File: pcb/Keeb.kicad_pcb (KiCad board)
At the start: 2 copper layers, 142.6 x 98.1 mm, 96 parts, among them J1 TRRS_SJ1-42514, J2 TRRS_SJ1-42514, K00 KEYSW, K01 KEYSW, K02 KEYSW, K03 KEYSW, K04 KEYSW, K05 KEYSW, K10 KEYSW, K11 KEYSW, K12 KEYSW, K13 KEYSW, K14 KEYSW, K15 KEYSW, K20 KEYSW, K21 KEYSW, K22 KEYSW, K23 KEYSW, K24 KEYSW, K25 KEYSW, K26 KEYSW, K30 KEYSW, K31 KEYSW, K32 KEYSW, K33 KEYSW, K34 KEYSW, K35 KEYSW, K36 KEYSW, SW1 SW_RST, U1 ATMEGA32U4, U2 PI6ULS5V9511AWEX_I2C_HotSwap, U3 MCP23017_SO, X1 XTAL_GND

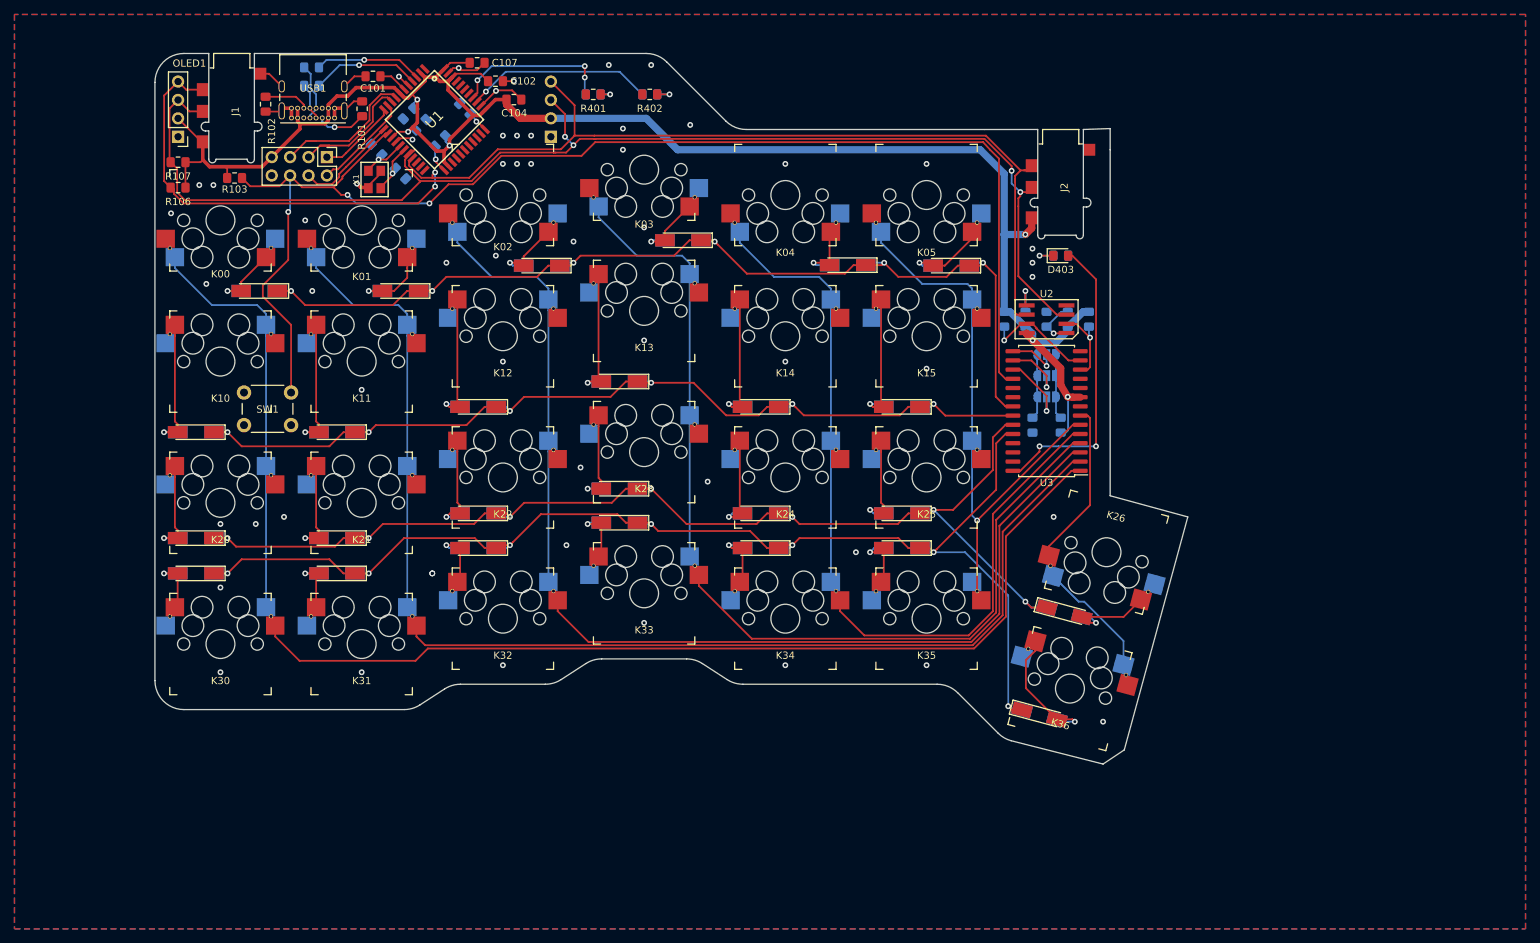
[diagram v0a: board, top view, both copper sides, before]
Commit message: restarted layout
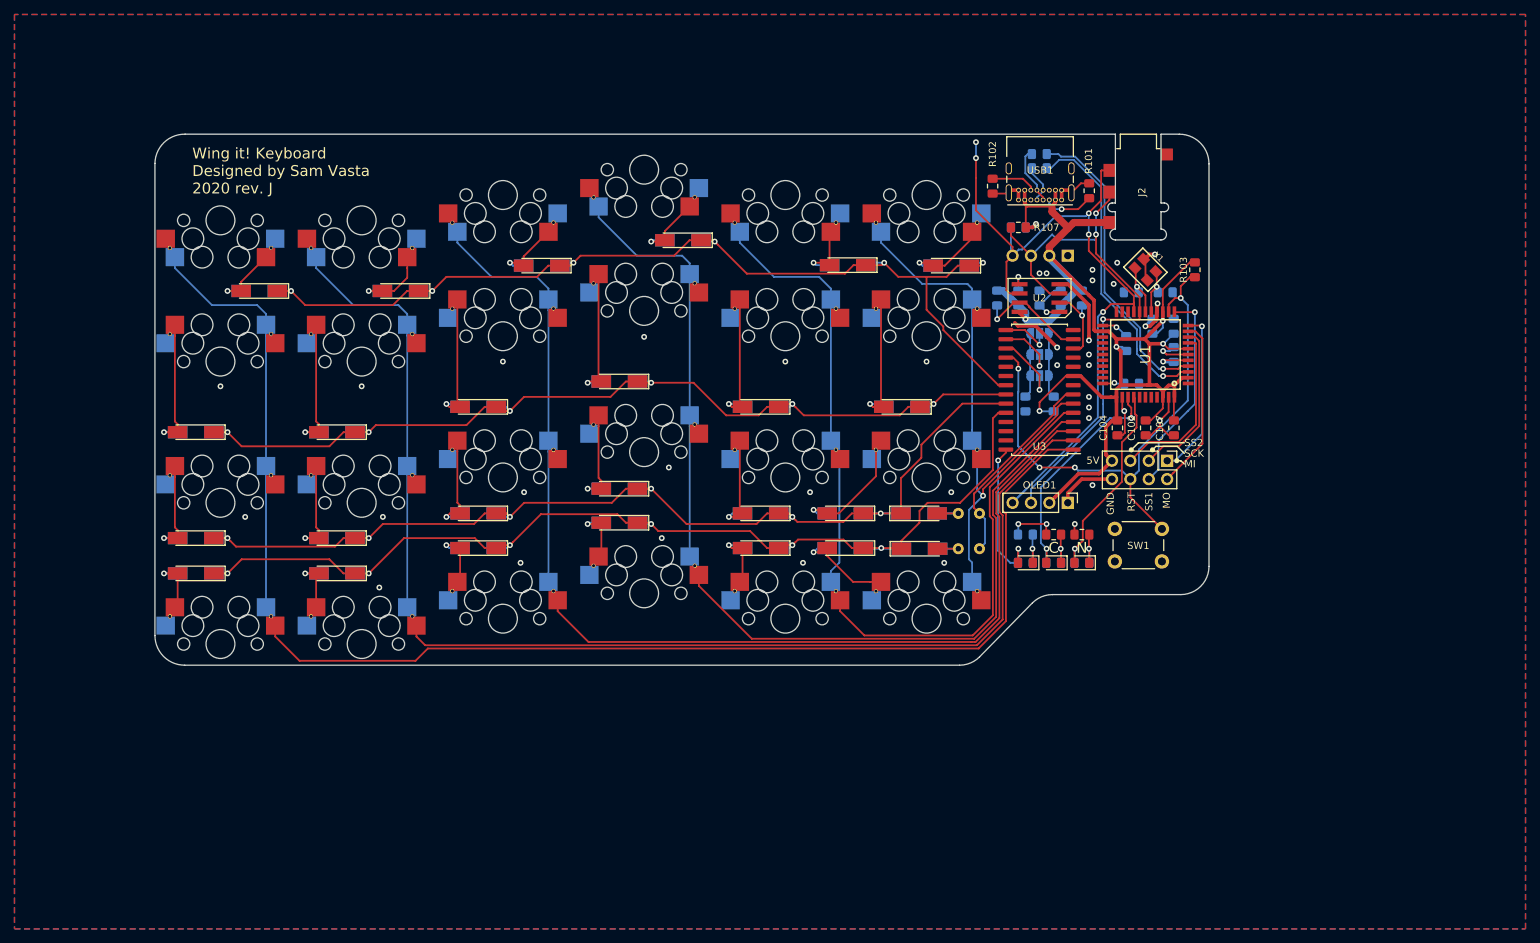
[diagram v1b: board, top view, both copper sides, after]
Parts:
- removed J1: TRRS_SJ1-42514, SVastaCustomParts:3.5mm_Cut_out
- removed JP0, JP1, JP2: SolderJumper_3_Open, Jumper:SolderJumper-3_P1.3mm_Open_RoundedPad1.0x1.5mm
- removed the OLED1 at (201.1, 43.2)
- removed the OLED1 at (252.5, 43.2)
- added 1: SolderJumper_3_Open, Jumper:SolderJumper-3_P1.3mm_Open_RoundedPad1.0x1.5mm, B.Cu at (320.0, 70.4)
- added 2: SolderJumper_3_Open, Jumper:SolderJumper-3_P1.3mm_Open_RoundedPad1.0x1.5mm, B.Cu at (320.0, 73.3)
- added 4: SolderJumper_3_Open, Jumper:SolderJumper-3_P1.3mm_Open_RoundedPad1.0x1.5mm, B.Cu at (320.0, 76.2)
- added D401: CAPS, LED_SMD:LED_0805_2012Metric_Pad1.15x1.40mm_HandSolder, F.Cu at (325.9, 102.0)
- added D402: NUM, LED_SMD:LED_0805_2012Metric_Pad1.15x1.40mm_HandSolder, F.Cu at (322.0, 102.0)
- added D403: CONN, LED_SMD:LED_0805_2012Metric_Pad1.15x1.40mm_HandSolder, B.Cu at (318.1, 102.0)
- added G***: LOGO, SVastaCustomParts:wing_it_400dpi, B.Cu at (215.2, 48.9)
- added OLED1: Conn_01x04, Connector_PinHeader_2.54mm:PinHeader_1x04_P2.54mm_Vertical, B.Cu at (323.9, 59.6)
- added OLED1: Conn_01x04, Connector_PinHeader_2.54mm:PinHeader_1x04_P2.54mm_Vertical, F.Cu at (323.9, 93.8)
- C101, R106: moved to B.Cu
- K26, K36: footprint SVastaCustomParts:Kailh_socket_reversible -> SVastaCustomParts:switch_off_board
- moved R103 133.2 mm to (341.5, 61.6), turned to 270 degrees
- moved SPI1 123.4 mm to (337.6, 87.9)
- moved SW1 118.2 mm to (333.7, 99.6)
- moved C101 117.0 mm to (338.5, 73.3), turned to 270 degrees
- moved R107 116.4 mm to (317.1, 55.7)
- moved R106 116.2 mm to (317.1, 55.7)
- moved C108 110.7 mm to (337.4, 64.7), turned to 0 degrees
- moved C106 109.7 mm to (338.5, 69.4), turned to 90 degrees
- moved C107 108.6 mm to (338.6, 83.4), turned to 270 degrees
- moved X1 107.2 mm to (334.6, 61.6), turned to 135 degrees
- moved C105 104.8 mm to (335.6, 69.4), turned to 90 degrees
- moved U1 103.4 mm to (334.6, 73.3), turned to 180 degrees
- moved C109 102.2 mm to (332.7, 64.7), turned to 180 degrees
- moved C102 101.7 mm to (334.7, 83.4), turned to 90 degrees
- moved R104 101.4 mm to (320.0, 47.6)
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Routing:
- net /RST: track 187.8 -> 76.9 mm, vias 3 -> 4
- net SCL: track 179.1 -> 79.2 mm, vias 4 -> 3
- net SDA: track 185.6 -> 105.9 mm, vias 2 -> 5
- net VCC: track 248.1 -> 175.4 mm
- net GND: track 45.4 -> 79.9 mm, vias 55 -> 42
- net Net-(R104-Pad1): track 14.9 -> 43.4 mm
- net Net-(R105-Pad1): track 15.0 -> 43.4 mm
- net /SwitchMatrix/Row3: track 174.6 -> 147.1 mm, vias 7 -> 6
- net /SwitchMatrix/Row2: track 162.5 -> 142.4 mm, vias 7 -> 6
- net /IO_Connected: track 41.6 -> 22.3 mm
- net /SwitchMatrix/Col6: track 45.7 -> 28.5 mm
- net Net-(D36-Pad2): track 21.2 -> 5.72 mm, vias 1 -> 0
- net /SS2: track 14.6 -> 28.5 mm, vias 0 -> 1
- net /MISO: track 11.4 -> 23.1 mm, vias 0 -> 1
- net Net-(D26-Pad2): track 16.7 -> 5.84 mm, vias 1 -> 0
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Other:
- board size 142.6 x 98.1 mm -> 145.5 x 73.3 mm
- board text added: "0"
- board text added: "Wing it! Keyboard Designed by Sam Vasta 2020 rev. J"
- board text added: "module address"
